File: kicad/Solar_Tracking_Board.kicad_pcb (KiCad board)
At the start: 2 copper layers, 23 parts, among them J1 Barrel_Jack, J10 Conn_01x03, J11 Conn_01x02_Female, J12 Conn_01x03, J13 Conn_01x02_Female, J14 MOUNTING_HOLE, J15 MOUNTING_HOLE, J16 MOUNTING_HOLE, J17 MOUNTING_HOLE, J2 Conn_02x03_Odd_Even, J3 Stack-Header_01x06, J4 Stack-Header_01x08, J5 Screw_Terminal_01x02, J6 Screw_Terminal_01x02, J7 Stack-Header_01x10, J8 Stack-Header_01x08, J9 Screw_Terminal_01x02

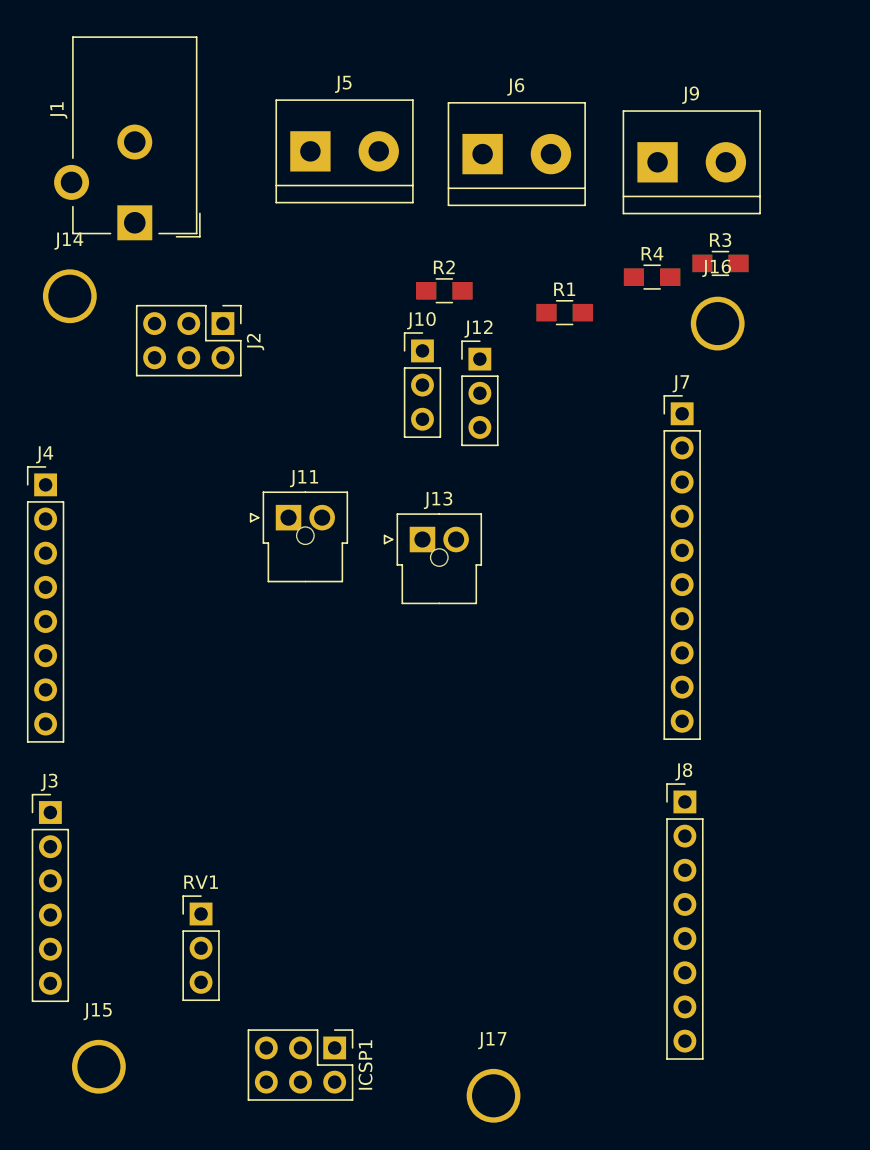
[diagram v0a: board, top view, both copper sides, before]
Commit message: Board Rev1 finsihed
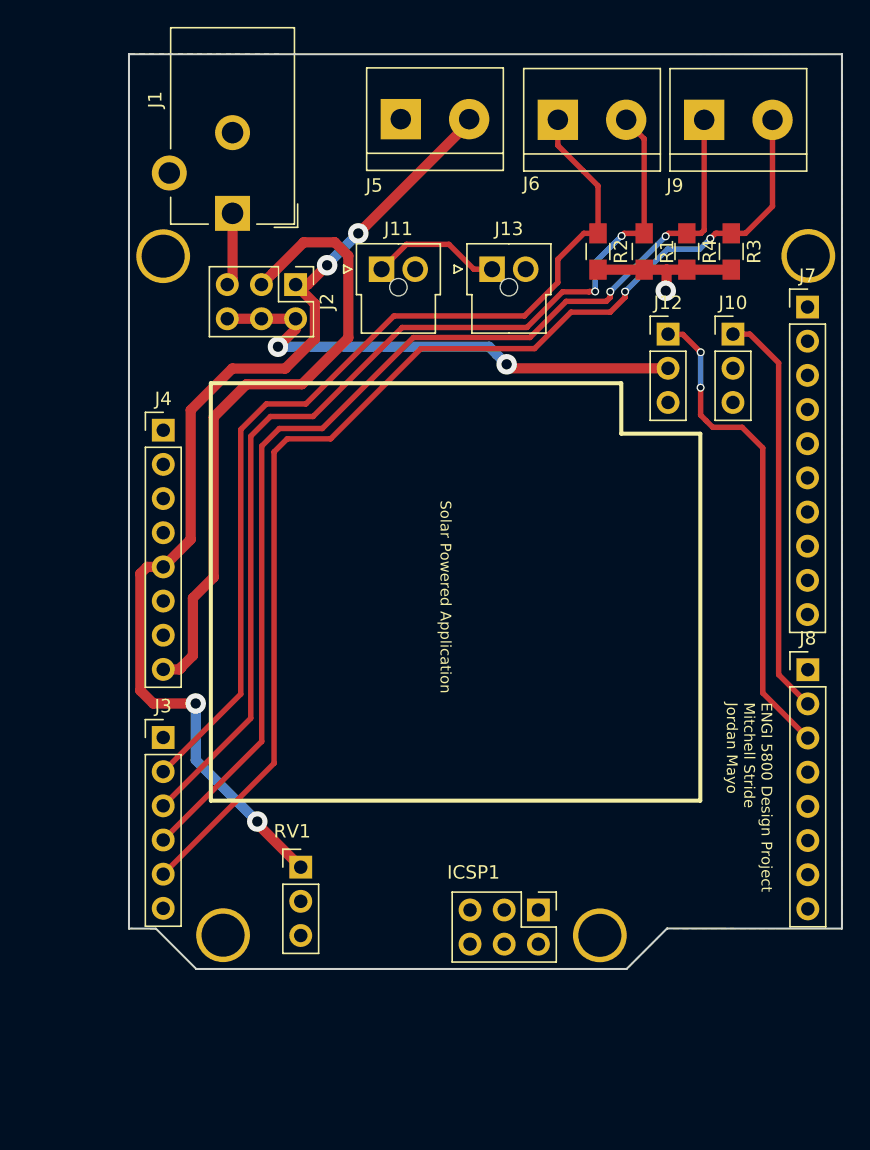
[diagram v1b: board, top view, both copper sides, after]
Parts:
- moved J10 23.1 mm to (157.0, 82.1)
- moved J13 20.7 mm to (139.1, 77.2)
- moved J11 19.7 mm to (130.9, 77.2)
- moved ICSP1 18.3 mm to (142.5, 124.9)
- moved J17 14.3 mm to (147.1, 126.8)
- moved J12 14.1 mm to (152.2, 82.1)
- moved J15 13.4 mm to (119.1, 126.7)
- moved J8 13.4 mm to (162.6, 107.0)
- moved J7 12.2 mm to (162.5, 80.1)
- moved R2 11.8 mm to (147.0, 75.9), turned to 270 degrees
- moved J3 10.1 mm to (114.6, 112.0)
- moved J4 9.64 mm to (114.6, 89.2)
- moved J16 8.41 mm to (162.6, 76.3)
- moved RV1 8.19 mm to (124.9, 121.7)
- moved J14 7.55 mm to (114.6, 76.3)
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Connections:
- J11 pad 1: (no net) -> SolarPWR_IN
- J13 pad 1: (no net) -> SolarPWR_IN
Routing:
- net A4: track 0.00 -> 86.1 mm, vias 0 -> 2
- net A3: track 0.00 -> 80.6 mm, vias 0 -> 2
- net +5V: track 0.00 -> 77.3 mm, vias 0 -> 4
- net A2: track 0.00 -> 75.9 mm, vias 0 -> 2
- net A1: track 0.00 -> 71.1 mm
- net Vin: track 0.00 -> 47.7 mm
- net Servo_PWR: track 0.00 -> 37.4 mm, vias 0 -> 2
- net 5: track 0.00 -> 36.2 mm, vias 0 -> 2
- net 6: track 0.00 -> 30.5 mm
- net GND: track 0.00 -> 11.5 mm, vias 0 -> 1
- net SolarPWR_IN: track 0.00 -> 9.75 mm
- net Barrel_PWR: track 0.00 -> 5.46 mm
- added copper zone on B.Cu, net GND
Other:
- board outline added: 53 x 68 mm
- net class PWR added: clearance 0.254, trace_width 0.762, via_dia 1.524, via_drill 0.762
- net class Signal added: clearance 0.254, trace_width 0.4064, via_dia 0.8128, via_drill 0.4064
- board text added: "ENGI 5800 Design Project Mitchell Stride Jordan Mayo"
- board text added: "Solar Powered Application"
